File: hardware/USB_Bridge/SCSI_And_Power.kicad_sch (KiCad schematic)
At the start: 20 parts, among them J10 BergFloppy, J3 DB25_Plug_MountingHoles, J7 TERM_BCKF, J8 EPWR

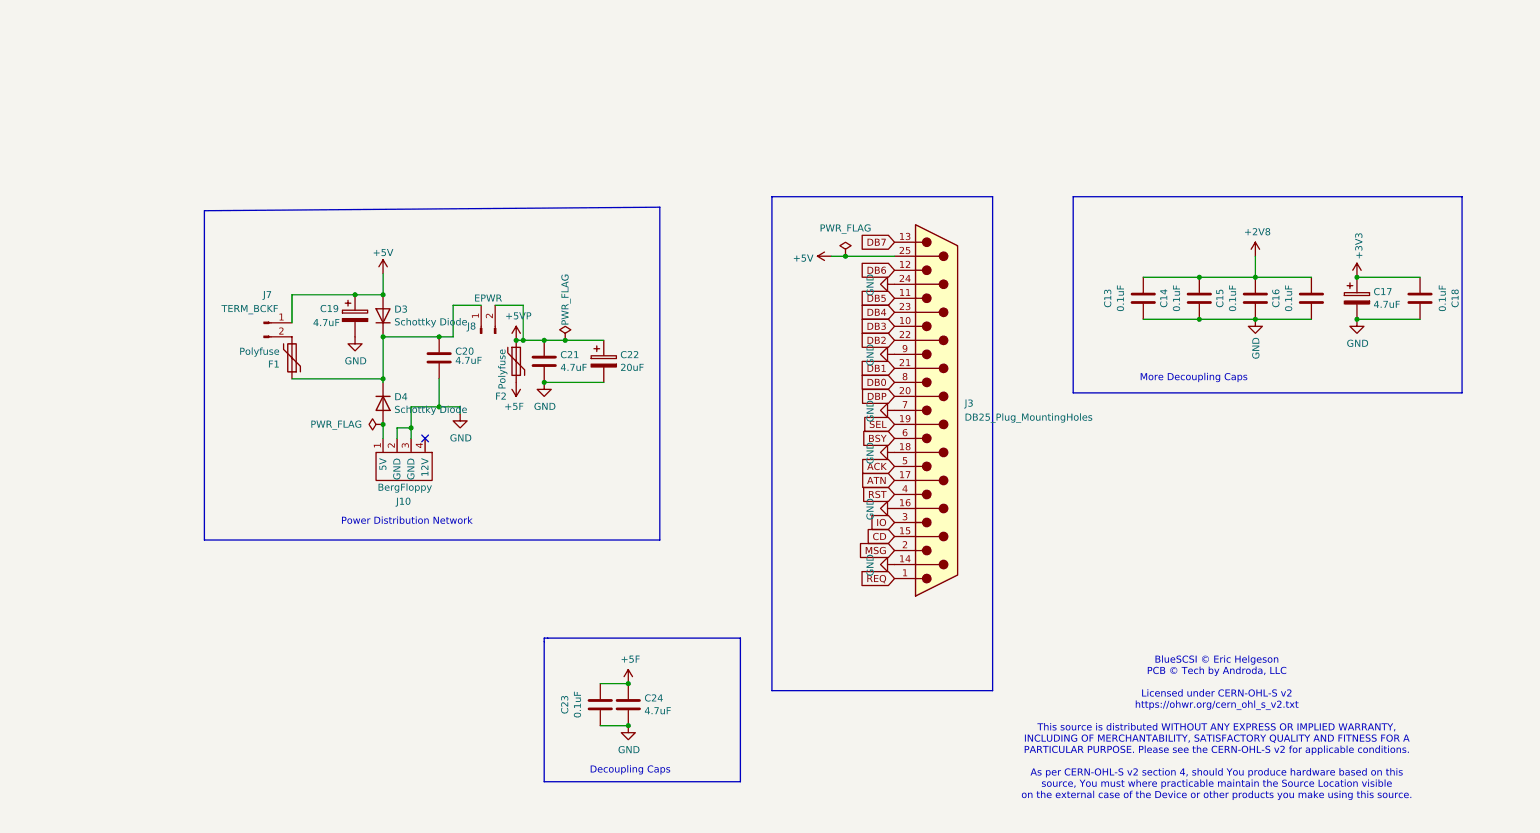
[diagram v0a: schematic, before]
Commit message: as-ordered PROTOTYPE
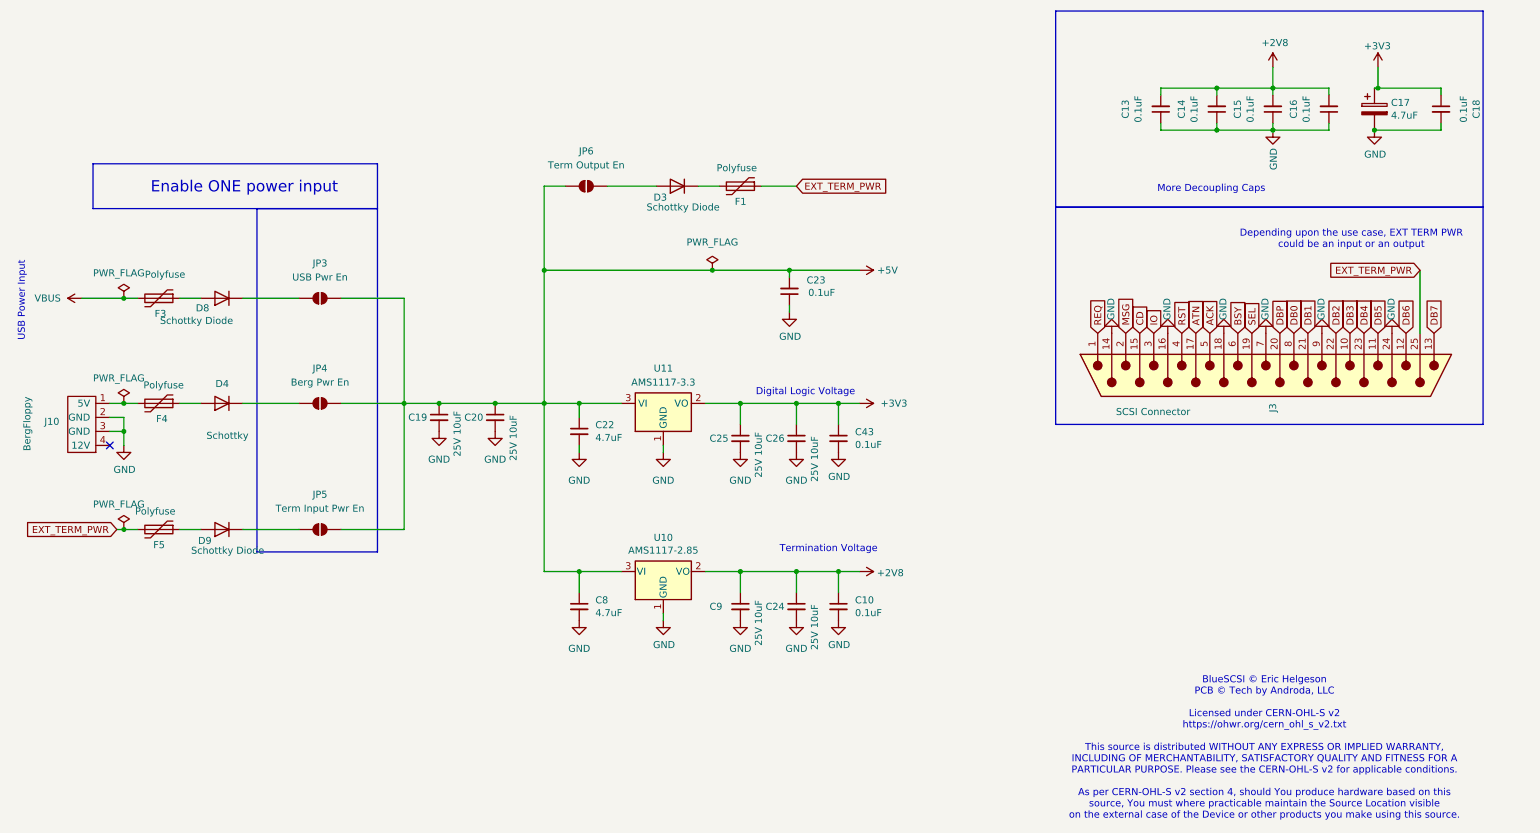
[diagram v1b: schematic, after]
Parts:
- removed C19: 4.7uF, Capacitor_SMD:C_0603_1608Metric, symbol Device:CP
- removed C20, C21, C24: 4.7uF, Capacitor_SMD:C_0603_1608Metric, symbol Device:C
- removed C22: 20uF, Capacitor_SMD:C_0603_1608Metric, symbol Device:CP
- removed C23: 0.1uF, Capacitor_SMD:C_0402_1005Metric, symbol Device:C
- removed F2: Polyfuse, Fuse:Fuse_0805_2012Metric_Pad1.15x1.40mm_HandSolder, symbol Device:Polyfuse
- removed J7: TERM_BCKF, Jumper:SolderJumper-2_P1.3mm_Open_RoundedPad1.0x1.5mm, symbol Connector:Conn_01x02_Male
- removed J8: EPWR, Jumper:SolderJumper-2_P1.3mm_Open_RoundedPad1.0x1.5mm, symbol Connector:Conn_01x02_Male
- added C10, C23, C43: 0.1uF, Capacitor_SMD:C_0402_1005Metric, symbol Device:C_Small
- added C19, C20, C24, C25, C26, C9: 25V 10uF, Capacitor_SMD:C_0603_1608Metric, symbol Device:C_Small
- added C22, C8: 4.7uF, Capacitor_SMD:C_0603_1608Metric, symbol Device:C_Small
- added D8, D9: Schottky Diode, Diode_SMD:D_SOD-123, symbol Device:D
- added F3, F4, F5: Polyfuse, Fuse:Fuse_0805_2012Metric_Pad1.15x1.40mm_HandSolder, symbol Device:Polyfuse
- added JP3: USB Pwr En, Jumper:SolderJumper-2_P1.3mm_Open_TrianglePad1.0x1.5mm, symbol Jumper:SolderJumper_2_Open
- added JP4: Berg Pwr En, Jumper:SolderJumper-2_P1.3mm_Open_TrianglePad1.0x1.5mm, symbol Jumper:SolderJumper_2_Open
- added JP5: Term Input Pwr En, Jumper:SolderJumper-2_P1.3mm_Open_TrianglePad1.0x1.5mm, symbol Jumper:SolderJumper_2_Open
- added JP6: Term Output En, Jumper:SolderJumper-2_P1.3mm_Open_TrianglePad1.0x1.5mm, symbol Jumper:SolderJumper_2_Open
- added U10: AMS1117-2.85, Package_TO_SOT_SMD:SOT-223-3_TabPin2, symbol Regulator_Linear:AMS1117CD-2.85
- added U11: AMS1117-3.3, Package_TO_SOT_SMD:SOT-223-3_TabPin2, symbol Regulator_Linear:AMS1117-3.3
- C13, C14, C15, C16, C18: symbol Device:C -> Device:C_Small
- D4: value Schottky Diode -> Schottky
- J3: value DB25_Plug_MountingHoles -> SCSI Connector
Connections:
- net +2V8: now also C10.1, C24.1, C9.1, U10.2 (VO)
- net +3V3: now also C25.1, C26.1, C43.1, U11.2 (VO)
- net +5V: now also C19.1, C20.1, C22.1, C23.2, C8.1, JP3.2 (B), JP4.2 (B), JP5.2 (B), JP6.1 (A), U10.3 (VI), U11.3 (VI); no longer D3.2 (A), J3.25 (P25)
- net GND: now also C10.2, C19.2, C20.2, C22.2, C23.1, C24.2, C25.2, C26.2, C43.2, C8.2, C9.2, U10.1 (GND), U11.1 (GND)
- net at J10.1 (5V): now also F4.2; no longer D4.2 (A)
- net at F1.2: now also D3.1 (K)
- new net: D8.2 (A), F3.1
- new net: D8.1 (K), JP3.1 (A)
- new net: D9.1 (K), JP5.1 (A)
- new net: D9.2 (A), F5.1
- new net: D4.2 (A), F4.1
- new net: D4.1 (K), JP4.1 (A)
- new net: D3.2 (A), JP6.2 (B)
- new net EXT_TERM_PWR: F1.1, F5.2, J3.25 (P25)
- new net VBUS: F3.2
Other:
- note added: "Depending upon the use case, EXT TERM PWR could be an input or an output"
- note added: "Digital Logic Voltage"
- note added: "Enable ONE power input"
- note added: "Termination Voltage"
- note added: "USB Power Input"
- note removed: "Decoupling Caps"
- note removed: "Power Distribution Network"
- moved on the sheet: C13, C14, C15, C16, C17, C18, D4, J10, J3
